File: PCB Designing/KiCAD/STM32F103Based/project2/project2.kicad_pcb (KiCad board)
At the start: 2 copper layers, 40 x 40 mm, 52 parts, among them J1 TYPE_C_31_M_12, J2 PLAY_BUTTON, J3 BATT, J8 Conn_02x06_Counter_Clockwise, Q1 AO3400A, SW1 BOOT, SW2 NRST, U1 BQ24074RGT, U2 LSM6DS3TR-C, U3 USBLC6-2SC6, U4 AP2112K-3.3, U5 ESP32-C3-WROOM-02

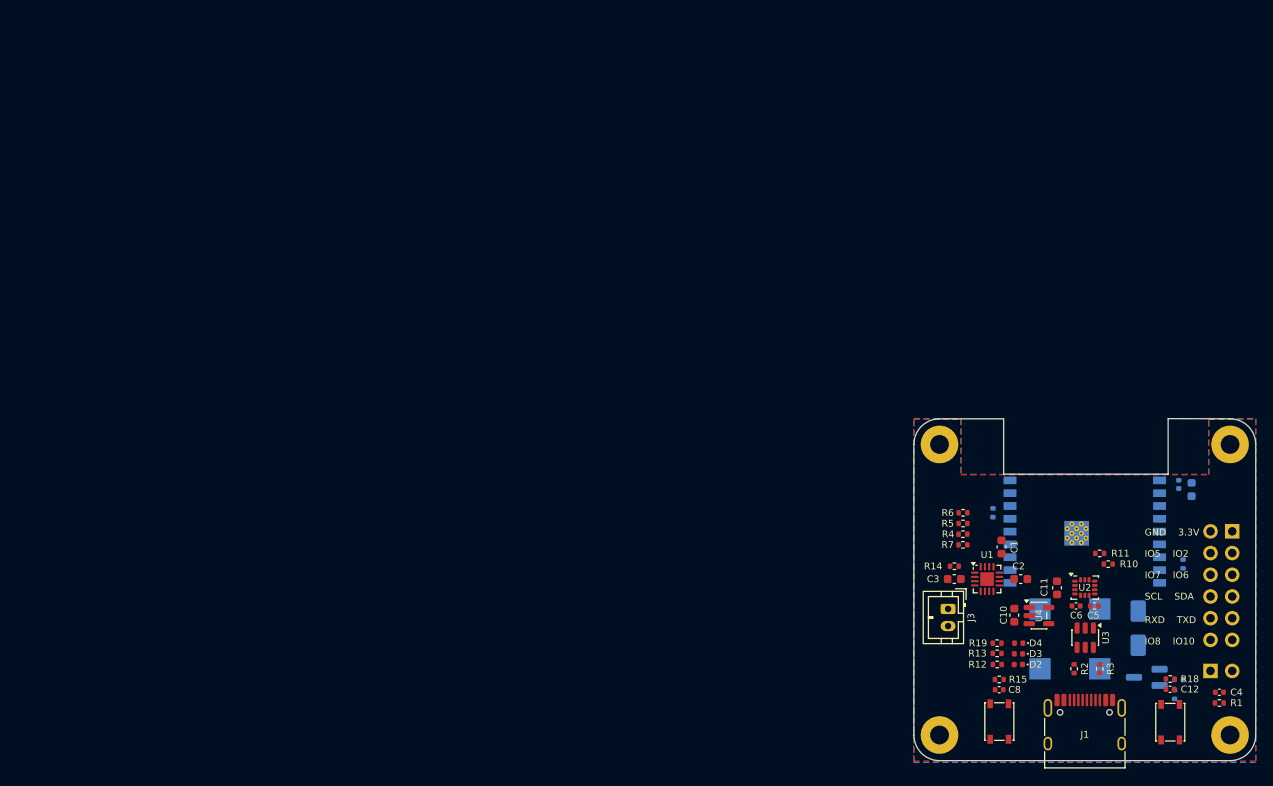
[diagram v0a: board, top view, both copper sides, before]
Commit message: Routing Alpha Draft
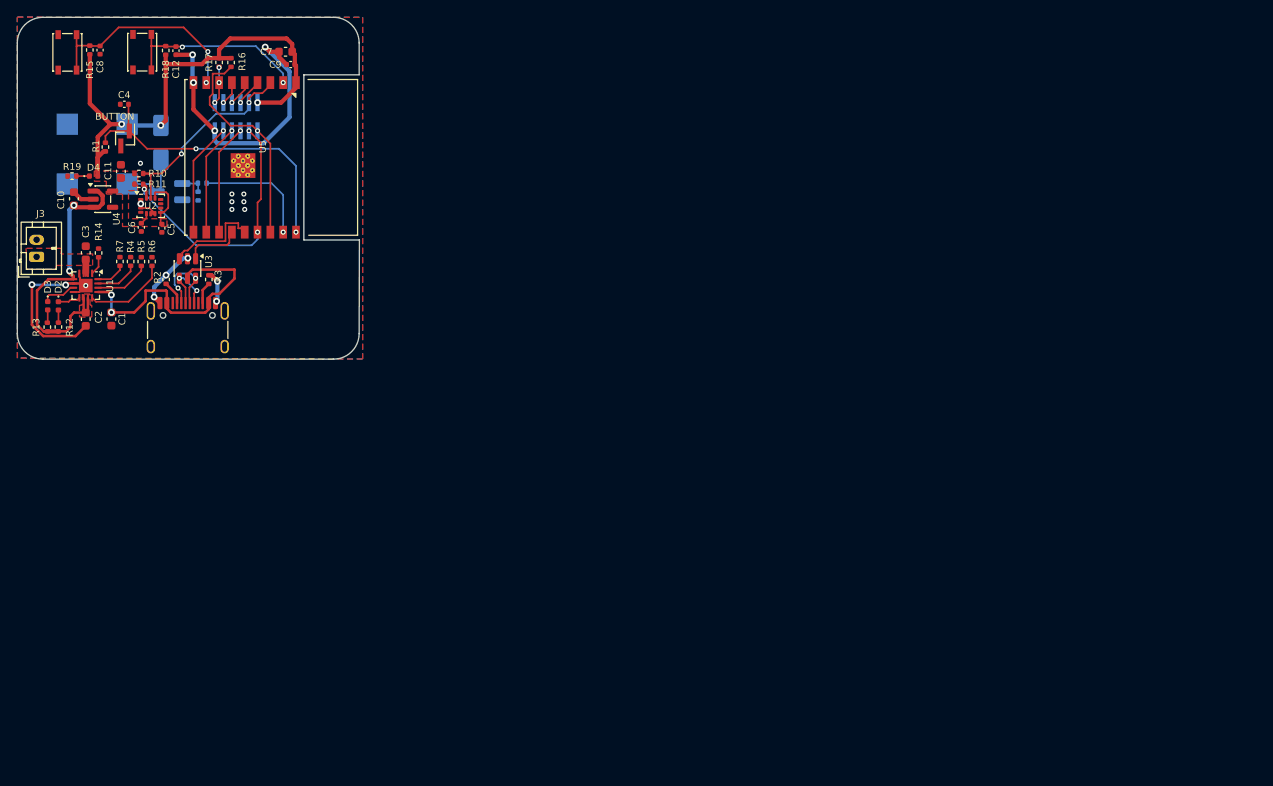
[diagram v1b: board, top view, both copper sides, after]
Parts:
- removed H1, H2, H3, H4: MountingHole, MountingHole:MountingHole_2.2mm_M2_Pad
- C7, C9, R16, R17, U5: moved to F.Cu
- J2: footprint Connector_PinHeader_2.54mm:PinHeader_1x02_P2.54mm_Vertical -> Connector_PinHeader_1.00mm:PinHeader_1x02_P1.00mm_Vertical_SMD_Pin1Left; moved to F.Cu
- J8: footprint Connector_PinHeader_2.54mm:PinHeader_2x06_P2.54mm_Vertical -> Connector_PinHeader_1.00mm:PinHeader_2x06_P1.00mm_Vertical_SMD
- moved R1 145.7 mm to (61.9, 54.2), turned to -90 degrees
- moved C4 145.4 mm to (64.1, 49.2), turned to 180 degrees
- moved SW2 143.6 mm to (66.2, 43.1)
- moved J2 141.5 mm to (64.2, 53.2)
- moved R18 138.7 mm to (69.0, 42.9), turned to -90 degrees
- moved C12 138.3 mm to (70.2, 42.9), turned to -90 degrees
- moved SW1 134.2 mm to (57.5, 43.1)
- moved R15 129.4 mm to (60.1, 42.8), turned to -90 degrees
- moved C8 129.1 mm to (61.3, 42.9), turned to -90 degrees
- moved R9 128.3 mm to (72.7, 59.9)
- moved R8 128.2 mm to (73.2, 58.4)
- moved D1 127.7 mm to (68.4, 53.7)
- moved Q1 127.7 mm to (69.4, 59.4)
- moved BZ1 127.2 mm to (60.9, 55.0)
- moved R17 127.2 mm to (75.2, 44.3), turned to 90 degrees
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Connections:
- J8 pad 1: +3.3V -> /IO2
- J8 pad 10: /RXD -> /IO7
- J8 pad 11: /IO10 -> GND
- J8 pad 2: GND -> +3.3V
- J8 pad 3: /IO2 -> /I2C_SDA
- J8 pad 4: /IO5 -> /I2C_SCL
- J8 pad 5: /IO6 -> /TXD
- J8 pad 6: /IO7 -> /IO5
- J8 pad 7: /I2C_SDA -> /RXD
- J8 pad 8: /I2C_SCL -> /IO6
- J8 pad 9: /TXD -> /IO10
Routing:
- net GND: track 0.00 -> 76.4 mm, vias 0 -> 20
- net +3.3V: track 0.00 -> 70.6 mm, vias 0 -> 3
- net /PLAY_BUTTON_MCU: track 0.00 -> 35.9 mm, vias 0 -> 2
- net VSYS: track 0.00 -> 35.1 mm, vias 0 -> 2
- net /I2C_SDA: track 0.00 -> 33.0 mm, vias 0 -> 3
- net VBUS: track 0.00 -> 31.8 mm, vias 0 -> 2
- net /IO2: track 0.00 -> 25.6 mm, vias 0 -> 1
- net /BOOT: track 0.00 -> 25.3 mm, vias 0 -> 2
- net /I2C_SCL: track 0.00 -> 24.2 mm, vias 0 -> 2
- net /CHIP_EN: track 0.00 -> 22.1 mm, vias 0 -> 2
- net /BUZZER_MCU: track 0.00 -> 13.9 mm, vias 0 -> 1
- net /IO10: track 0.00 -> 13.3 mm, vias 0 -> 1
- net /RXD: track 0.00 -> 13.1 mm, vias 0 -> 1
- net /TXD: track 0.00 -> 12.9 mm, vias 0 -> 1
- net /MCU_USB_D_P: track 0.00 -> 11.6 mm
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- added copper zone on F.Cu, net +3.3V
- added copper zone on F.Cu, net +BATT
- added copper zone on F.Cu, net VSYS
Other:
- outline, holes or cut-outs redrawn
- board text removed: "GND 3.3V"
- board text removed: "IO5 IO2"
- board text removed: "IO7 IO6"
- board text removed: "IO8 IO10"
- board text removed: "RXD TXD"
- board text removed: "SCL SDA"
